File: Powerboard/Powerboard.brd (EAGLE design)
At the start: 87.5 x 150 mm, 11 parts

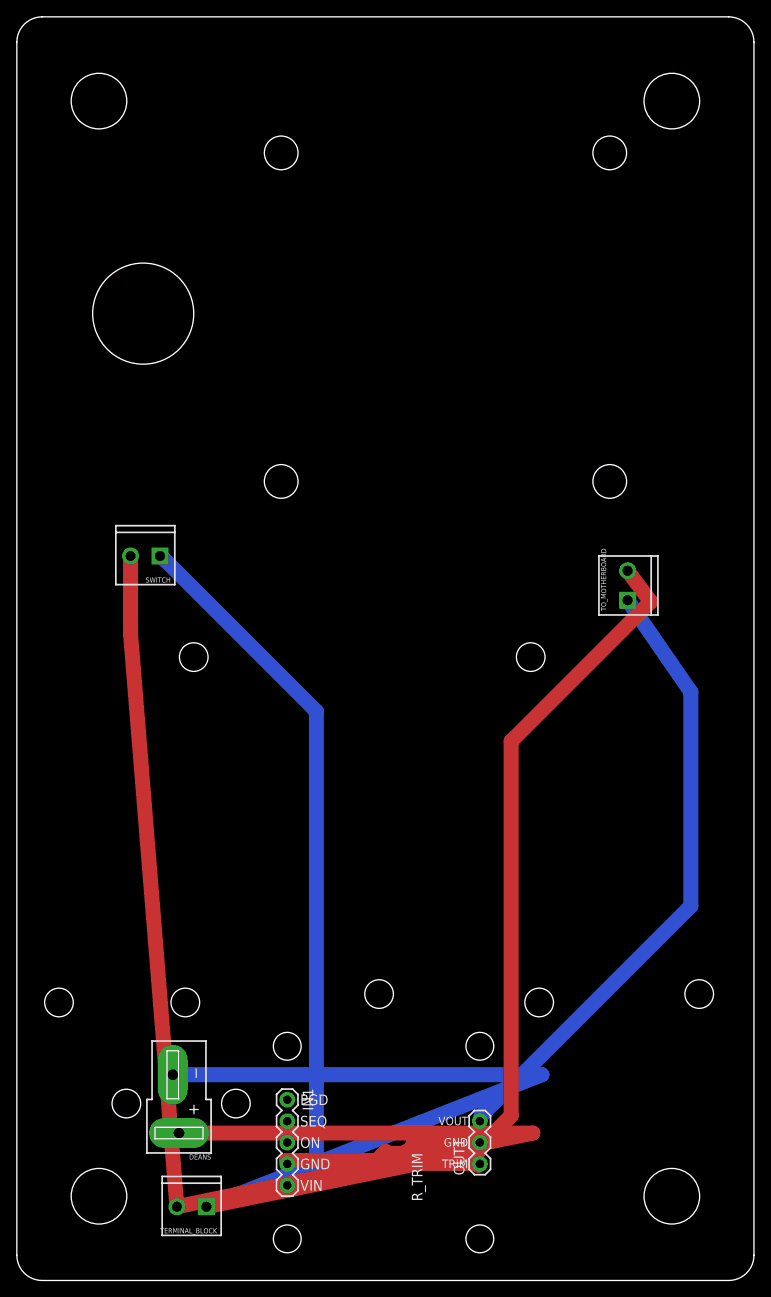
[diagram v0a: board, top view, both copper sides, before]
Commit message: layout r2
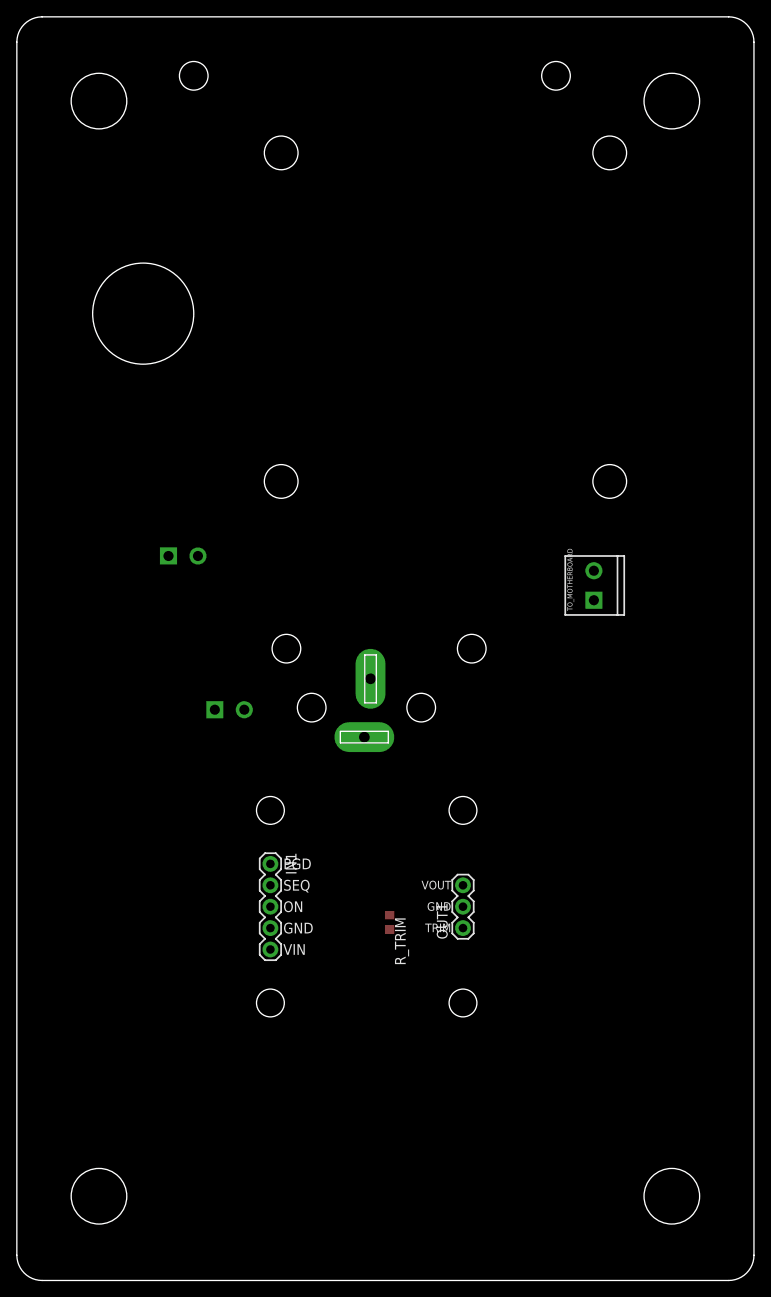
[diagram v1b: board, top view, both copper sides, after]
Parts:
- removed TERMINAL_BLOCK: (no value), SparkFun-Connectors:SCREWTERMINAL-3.5MM-2
- added BATTERY_TERMINAL_BLOCK: (no value), SparkFun-Connectors:SCREWTERMINAL-3.5MM-2
- moved DEANS 51.9 mm to (41.2, 64.5), flipped to the bottom
- moved IN1 28.1 mm to (30.1, 49.5)
- moved OUT1 28.1 mm to (53.0, 41.8)
- moved R_TRIM 28.1 mm to (44.2, 42.5)
- moved U$2 28.1 mm to (30.1, 55.8)
- moved U$6 28.1 mm to (30.1, 32.9)
- moved U$7 28.1 mm to (53.0, 55.8)
- moved U$8 28.1 mm to (53.0, 32.9)
- moved TO_MOTHERBOARD 4.00 mm to (68.5, 80.8)
- moved SWITCH 1.00 mm to (18.0, 86.0), flipped to the bottom
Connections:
- net GND: now also BATTERY_TERMINAL_BLOCK.1, TO_MOTHERBOARD.1; no longer TERMINAL_BLOCK.1, TO_MOTHERBOARD.2
- net N$1: now also BATTERY_TERMINAL_BLOCK.2; no longer TERMINAL_BLOCK.2
- net VOUT: now also TO_MOTHERBOARD.2; no longer TO_MOTHERBOARD.1
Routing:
- net GND: track 230.4 -> 0.00 mm
- net N$1: track 162.6 -> 0.00 mm
- net VIN: track 85.2 -> 0.00 mm
- net VOUT: track 74.5 -> 0.00 mm
- net TRIM: track 8.78 -> 0.00 mm
